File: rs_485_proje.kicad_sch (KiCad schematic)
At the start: 61 parts, among them J11 P_E_SENSOR_1, J12 P_E_SENSOR_2, J2 RJ45_LED, J4 Led_conn, J6 USB_B_Mini, J7 H_E_sensor_1, J8 H_E_sensor_2, J9 Debug, U1 AP2112K-3.3, U10 FT232RL, U11 USBLC6-2SC6, U2 STM32G030F6Px, U4 ADM2587E, U5 TPS5420D, U7 TLP2161

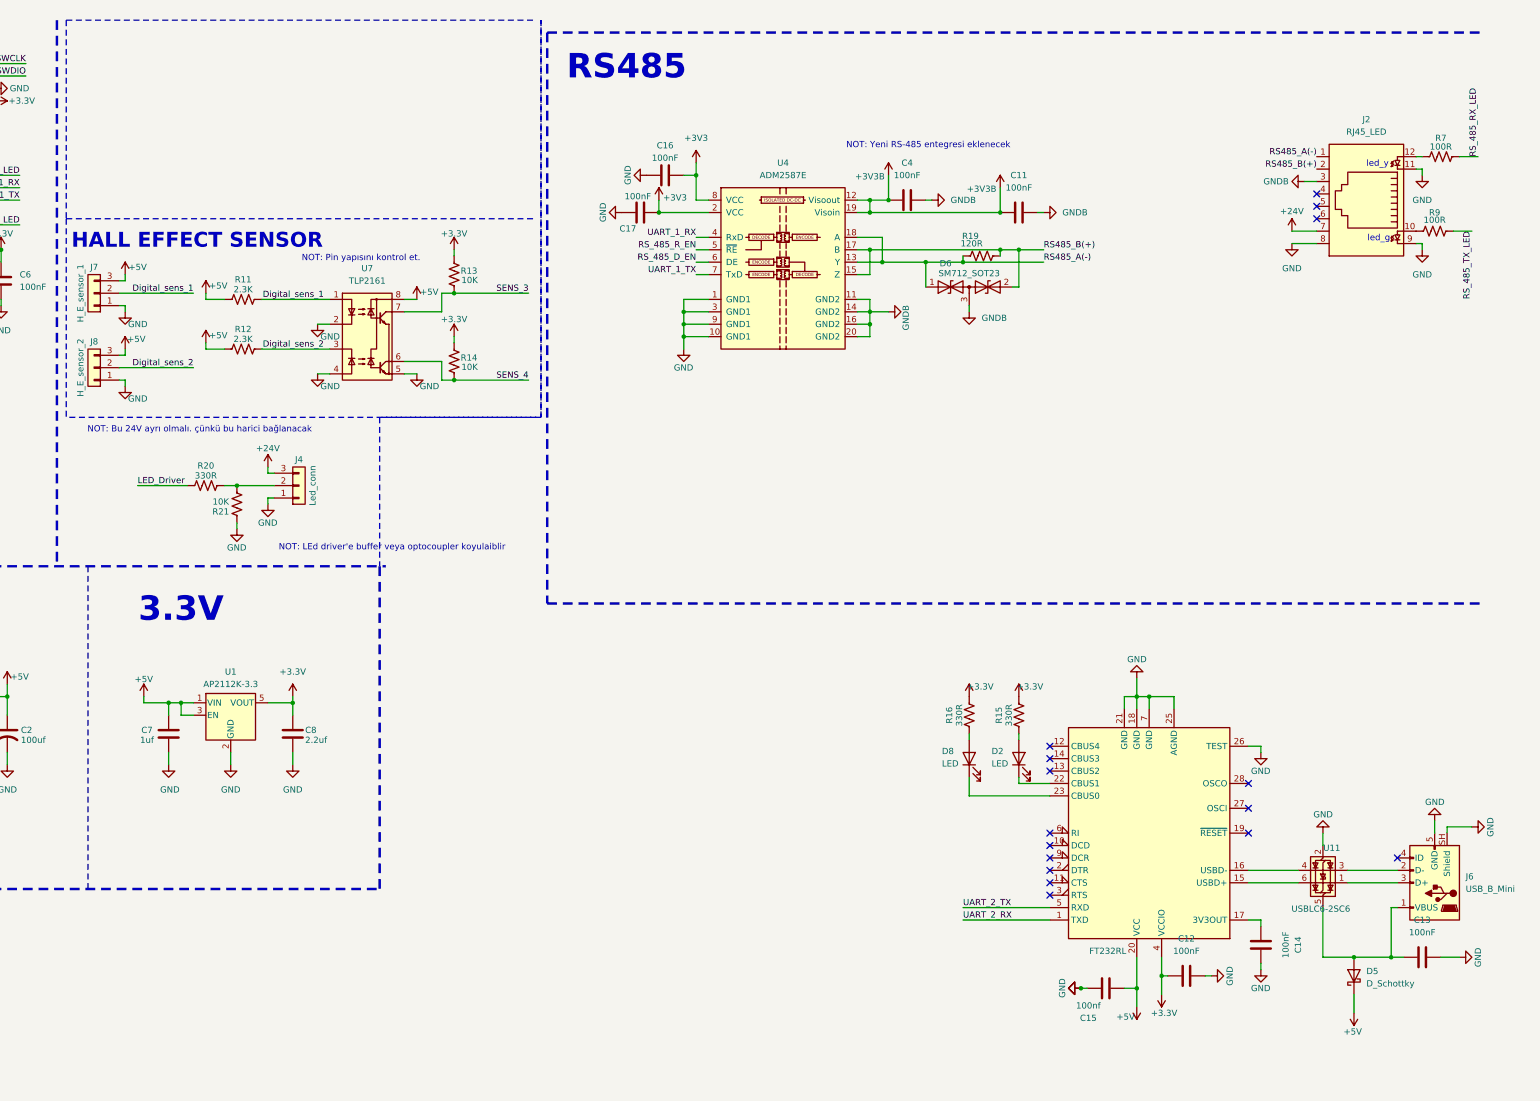
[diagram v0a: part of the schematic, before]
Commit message: 27/04/15:17
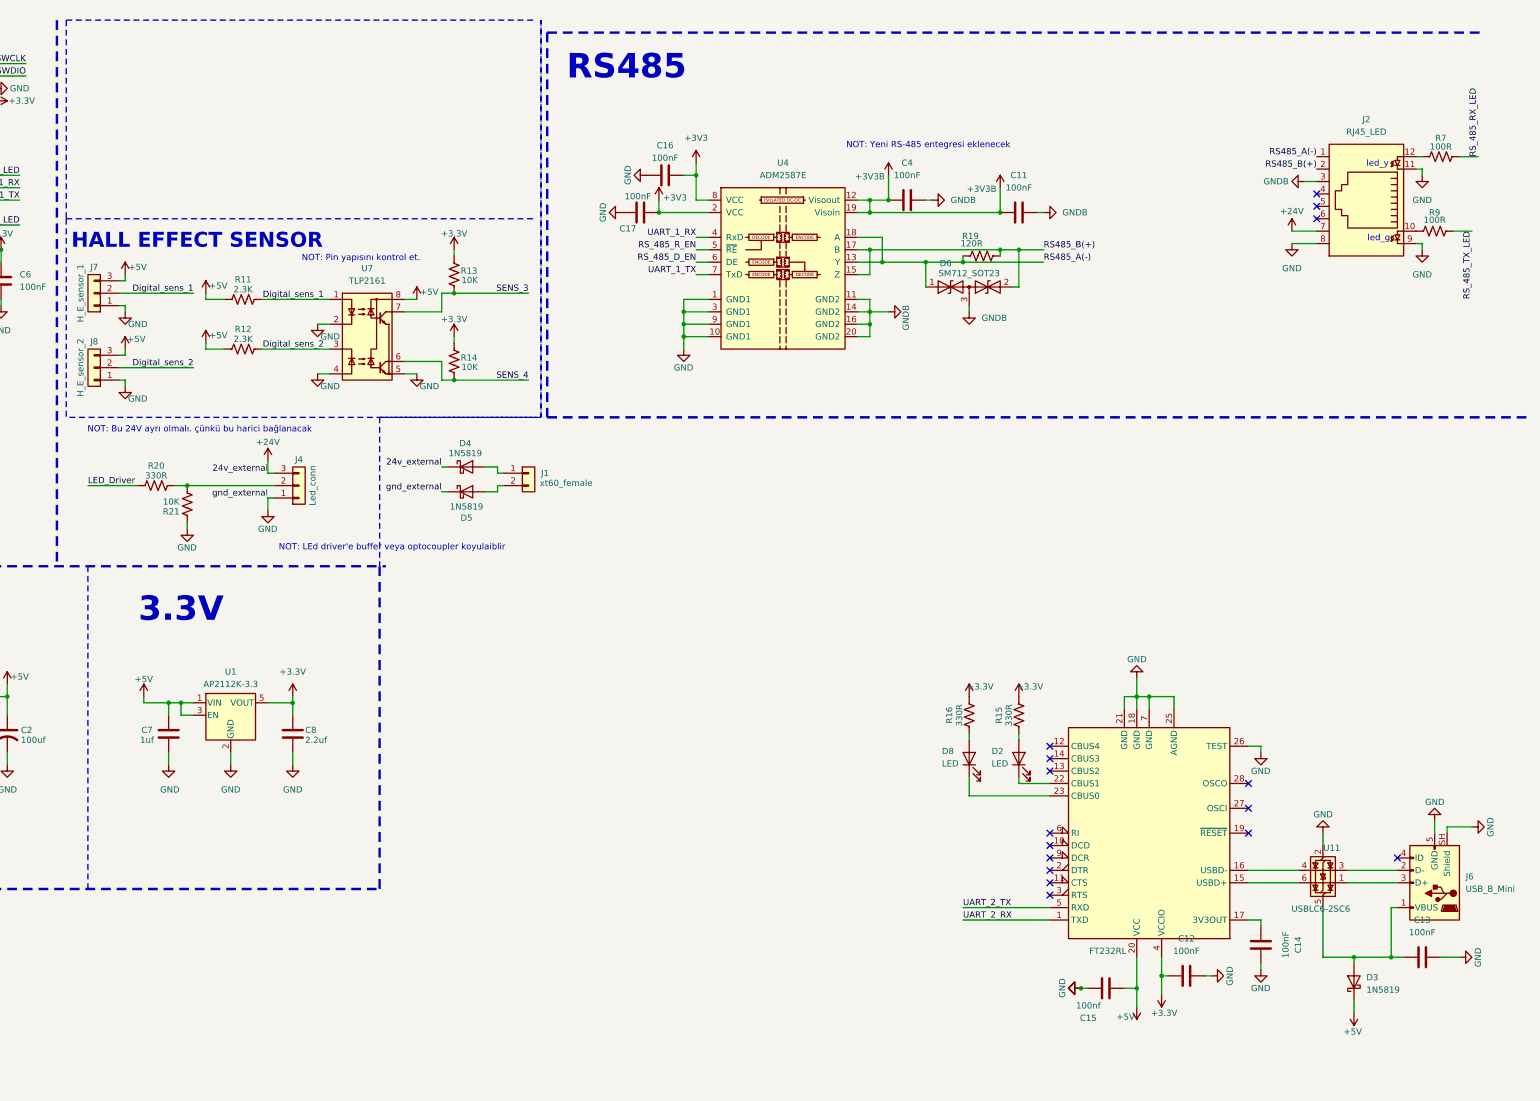
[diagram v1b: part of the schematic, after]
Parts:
- removed D5: D_Schottky, symbol Device:D_Schottky
- added D3, D4, D5: 1N5819, Diode_THT:D_DO-41_SOD81_P10.16mm_Horizontal, symbol Diode:1N5819
- added J1: xt60_female, Connector_AMASS:AMASS_XT60-F_1x02_P7.20mm_Vertical, symbol Connector_Generic:Conn_01x02
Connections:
- net +24V: now also D4.1 (K)
- net +5V: now also D3.1 (K)
- net GND: now also D5.1 (K)
- net at C13.1, J6.1 (VBUS), U11.5 (VBUS): now also D3.2 (A)
- new net: D4.2 (A), J1.1 (Pin_1)
- new net: D5.2 (A), J1.2 (Pin_2)
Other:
- moved on the sheet: R20, R21
